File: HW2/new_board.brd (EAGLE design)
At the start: 50 x 50 mm, 22 parts, among them X1 HC49-HC49-3L

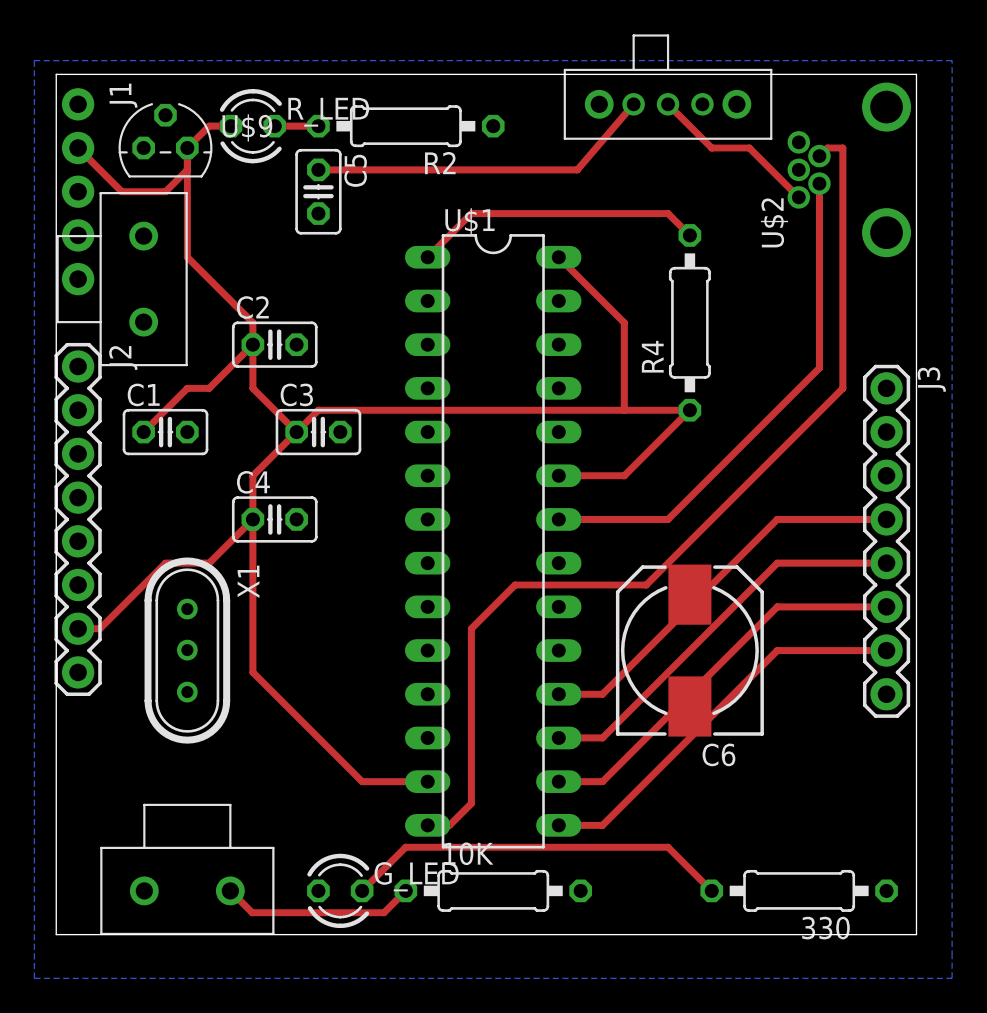
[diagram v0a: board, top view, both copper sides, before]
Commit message: board
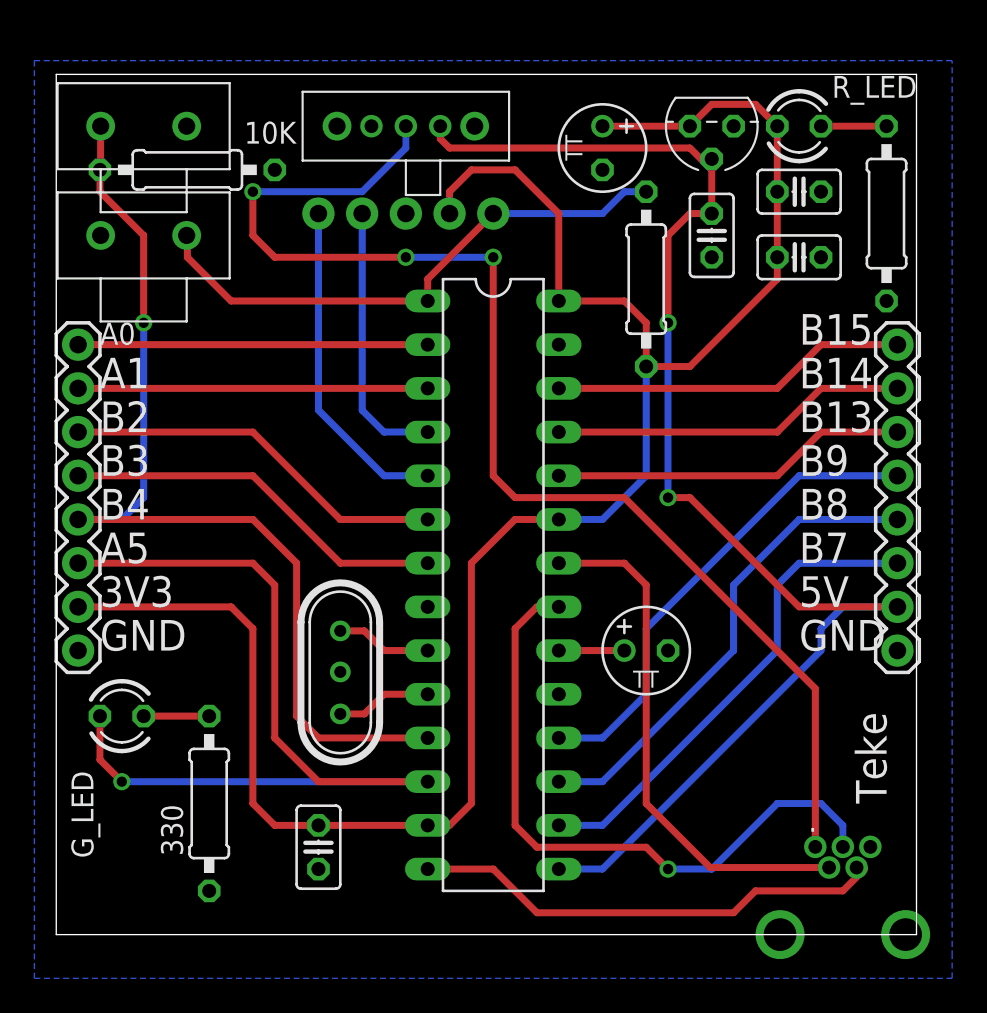
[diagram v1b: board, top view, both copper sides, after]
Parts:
- removed C2: 0.1uF, new_library:C025-025X050
- removed U$2: MINI_USB, new_library:USB-MB-H
- added .: MINI_USB, new_library:USB-MB-H
- added C7: 10uF, new_library:TT2D5
- C6: device new_library:150CLZ-0810 -> new_library:TT2D5
- moved 10K 45.5 mm to (7.62, 44.5)
- moved U$5 44.5 mm to (5.08, 47.0), turned to 180 degrees
- moved C1 39.4 mm to (43.2, 43.2)
- moved 330 34.7 mm to (8.89, 7.62), turned to 90 degrees
- moved U$9 31.8 mm to (38.1, 47.0), turned to 180 degrees
- moved R_LED 31.8 mm to (43.2, 47.0)
- moved C3 29.7 mm to (43.2, 39.4)
- moved R2 28.4 mm to (48.3, 41.9), turned to 90 degrees
- moved J1 25.0 mm to (25.4, 41.9), turned to 180 degrees
- moved C5 23.0 mm to (38.1, 40.6)
- moved C4 19.2 mm to (15.2, 5.08), turned to 270 degrees
- moved G_LED 16.3 mm to (3.81, 12.7)
- moved U$3 15.3 mm to (20.3, 47.0), turned to 180 degrees
- moved X1 8.98 mm to (16.5, 15.2)
- moved R4 3.59 mm to (34.3, 38.1)
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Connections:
- net +3V3: now also C7.+; no longer C2.1
- net GND: now also ..GND, C7.-; no longer C2.2, U$2.GND
- net N$1: now also ..ID; no longer U$2.ID
- net N$13: now also ..VBUS; no longer U$2.VBUS
- net N$15: now also ..D-; no longer U$2.D-
- net N$16: now also ..D+; no longer U$2.D+
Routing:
- net N$13: track 9.84 -> 74.0 mm, vias 0 -> 3
- net N$12: track 0.00 -> 52.9 mm, vias 0 -> 1
- net N$6: track 11.3 -> 57.8 mm, vias 0 -> 1
- net N$14: track 43.3 -> 81.4 mm, vias 0 -> 2
- net N$16: track 0.00 -> 38.0 mm, vias 0 -> 1
- net N$1: track 56.1 -> 28.0 mm
- net N$22: track 0.00 -> 22.4 mm
- net N$21: track 0.00 -> 22.4 mm
- net N$25: track 0.00 -> 20.7 mm
- net N$24: track 0.00 -> 20.7 mm
- net N$23: track 0.00 -> 20.7 mm
- net N$20: track 0.00 -> 20.3 mm
- net N$19: track 0.00 -> 20.3 mm
- net N$3: track 0.00 -> 19.4 mm
- net N$11: track 22.4 -> 3.81 mm
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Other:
- board text added: "3V3"
- board text added: "5V"
- board text added: "A0"
- board text added: "A1"
- board text added: "A5"
- board text added: "B13"
- board text added: "B14"
- board text added: "B15"
- board text added: "B2"
- board text added: "B3"
- board text added: "B4"
- board text added: "B7"
- board text added: "B8"
- board text added: "B9"
- board text added: "GND"
- board text added: "Teke"
